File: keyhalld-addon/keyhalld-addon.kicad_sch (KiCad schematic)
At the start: 66 parts, among them J1 Conn_01x06_Pin, J2 USB_C_Receptacle_USB2.0_16P, J3 Conn_01x04_Pin, SW1 SW_Push, SW10 RST, SW2 SW_Push, SW3 SW_Push, SW4 SW_Push, SW5 SW_Push, SW6 SW_Push, SW7 SW_Push, SW8 SW_Push, SW9 BOOT, U1 TLV1117-33, U2 RP2350A, U3 USBLC6-2SC6, U4 ER_OLEDM0.91_1x-I2C, Y1 12MHz

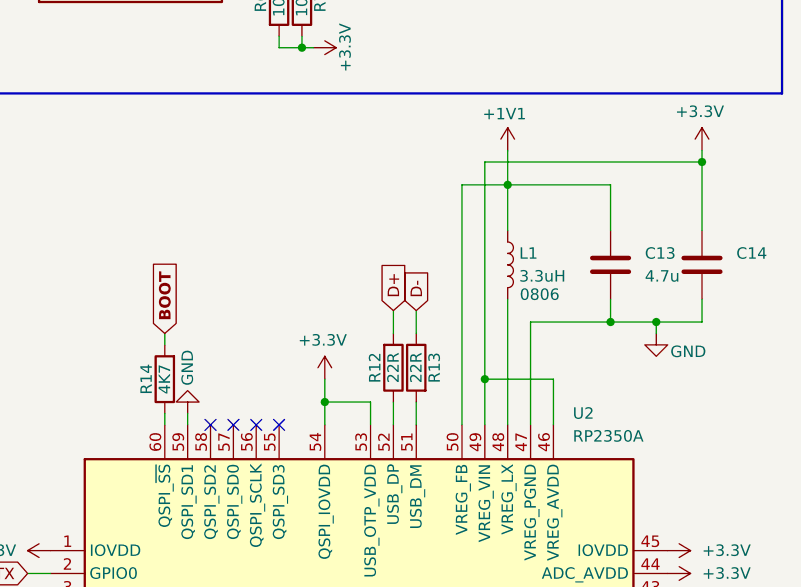
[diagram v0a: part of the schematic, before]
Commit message: routed pcb for addon board
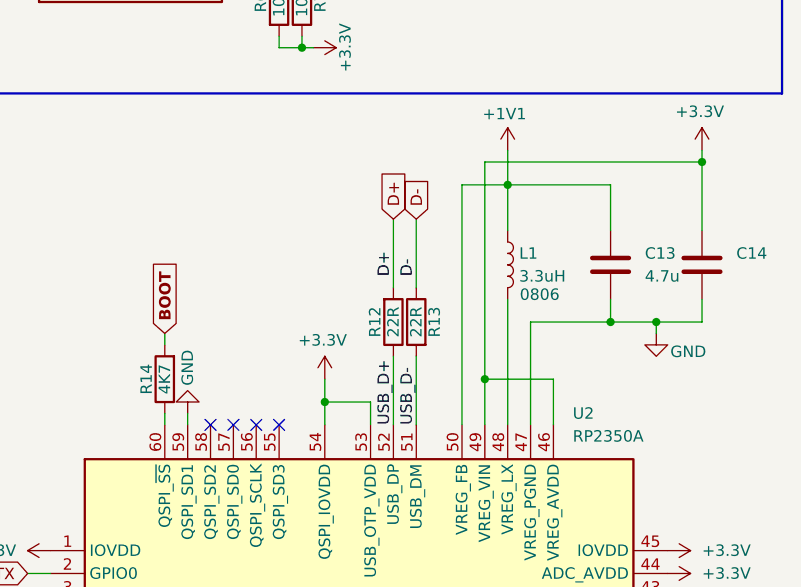
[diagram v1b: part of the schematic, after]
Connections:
- net USB_D-: now reaches R13.2, U2.51 (USB_DM)
- net USB_D+: now reaches R12.1, U2.52 (USB_DP)
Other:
- moved on the sheet: R12, R13
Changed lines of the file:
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@@
 	(wire
 		(pts
-			(xy 222.25 74.93) (xy 222.25 77.47)
+			(xy 222.25 64.77) (xy 222.25 72.39)
 		)
 		(stroke
@@
 	(wire
 		(pts
-			(xy 222.25 85.09) (xy 222.25 87.63)
+			(xy 222.25 80.01) (xy 222.25 87.63)
 		)
 		(stroke
@@
 	(wire
 		(pts
-			(xy 224.79 85.09) (xy 224.79 87.63)
+			(xy 224.79 80.01) (xy 224.79 87.63)
 		)
 		(stroke
@@
 	(wire
 		(pts
-			(xy 224.79 74.93) (xy 224.79 77.47)
+			(xy 224.79 64.77) (xy 224.79 72.39)
 		)
 		(stroke
@@
 		)
 	)
+	(label "USB_D-"
+		(at 224.79 87.63 90)
+		(effects
+			(font
+				(size 1.27 1.27)
+			)
+			(justify left bottom)
+		)
+	)
 	(label "CONN_D-"
 		(at 88.9 140.97 0)
@@
 		)
 	)
+	(label "USB_D+"
+		(at 222.25 87.63 90)
+		(effects
+			(font
+				(size 1.27 1.27)
+			)
+			(justify left bottom)
+		)
+	)
 	(label "CONN_D+"
 		(at 88.9 143.51 0)
@@
 		)
 	)
+	(label "D+"
+		(at 222.25 71.12 90)
+		(effects
+			(font
+				(size 1.27 1.27)
+			)
+			(justify left bottom)
+		)
+	)
+	(label "D-"
+		(at 224.79 71.12 90)
+		(effects
+			(font
+				(size 1.27 1.27)
+			)
+			(justify left bottom)
+		)
+	)
 	(global_label "WS_LED"
 		(shape input)
@@
 	(global_label "D+"
 		(shape input)
-		(at 222.25 74.93 90)
+		(at 222.25 64.77 90)
 		(fields_autoplaced yes)
 		(effects
@@
 		)
 		(property "Intersheetrefs" "${INTERSHEET_REFS}"
-			(at 222.25 69.1024 90)
+			(at 222.25 58.9424 90)
 			(hide yes)
 			(show_name no)
@@
 	(global_label "D-"
 		(shape input)
-		(at 224.79 74.93 90)
+		(at 224.79 64.77 90)
 		(fields_autoplaced yes)
 		(effects
@@
 		)
 		(property "Intersheetrefs" "${INTERSHEET_REFS}"
-			(at 224.79 69.1024 90)
+			(at 224.79 58.9424 90)
 			(hide yes)
 			(show_name no)
@@
 	(symbol
 		(lib_id "Device:R")
-		(at 224.79 81.28 0)
+		(at 224.79 76.2 0)
 		(mirror y)
 		(unit 1)
@@
 		(dnp no)
 		(property "Reference" "R13"
-			(at 226.822 81.28 90)
+			(at 226.822 76.2 90)
 			(show_name no)
 			(do_not_autoplace no)
@@
 		)
 		(property "Value" "22R"
-			(at 224.79 81.28 90)
+			(at 224.79 76.2 90)
 			(show_name no)
 			(do_not_autoplace no)
@@
 		)
 		(property "Footprint" "Resistor_SMD:R_0603_1608Metric_Pad0.98x0.95mm_HandSolder"
-			(at 226.568 81.28 90)
+			(at 226.568 76.2 90)
 			(hide yes)
 			(show_name no)
@@
 		)
 		(property "Datasheet" ""
-			(at 224.79 81.28 0)
+			(at 224.79 76.2 0)
 			(hide yes)
 			(show_name no)
@@
 		)
 		(property "Description" "Resistor"
-			(at 224.79 81.28 0)
+			(at 224.79 76.2 0)
 			(hide yes)
 			(show_name no)
@@
 	(symbol
 		(lib_id "Device:R")
-		(at 222.25 81.28 0)
+		(at 222.25 76.2 0)
 		(mirror x)
 		(unit 1)
@@
 		(dnp no)
 		(property "Reference" "R12"
-			(at 220.218 81.28 90)
+			(at 220.218 76.2 90)
 			(show_name no)
 			(do_not_autoplace no)
@@
 		)
 		(property "Value" "22R"
-			(at 222.25 81.28 90)
+			(at 222.25 76.2 90)
 			(show_name no)
 			(do_not_autoplace no)
@@
 		)
 		(property "Footprint" "Resistor_SMD:R_0603_1608Metric_Pad0.98x0.95mm_HandSolder"
-			(at 220.472 81.28 90)
+			(at 220.472 76.2 90)
 			(hide yes)
 			(show_name no)
@@
 		)
 		(property "Datasheet" ""
-			(at 222.25 81.28 0)
+			(at 222.25 76.2 0)
 			(hide yes)
 			(show_name no)
@@
 		)
 		(property "Description" "Resistor"
-			(at 222.25 81.28 0)
+			(at 222.25 76.2 0)
 			(hide yes)
 			(show_name no)

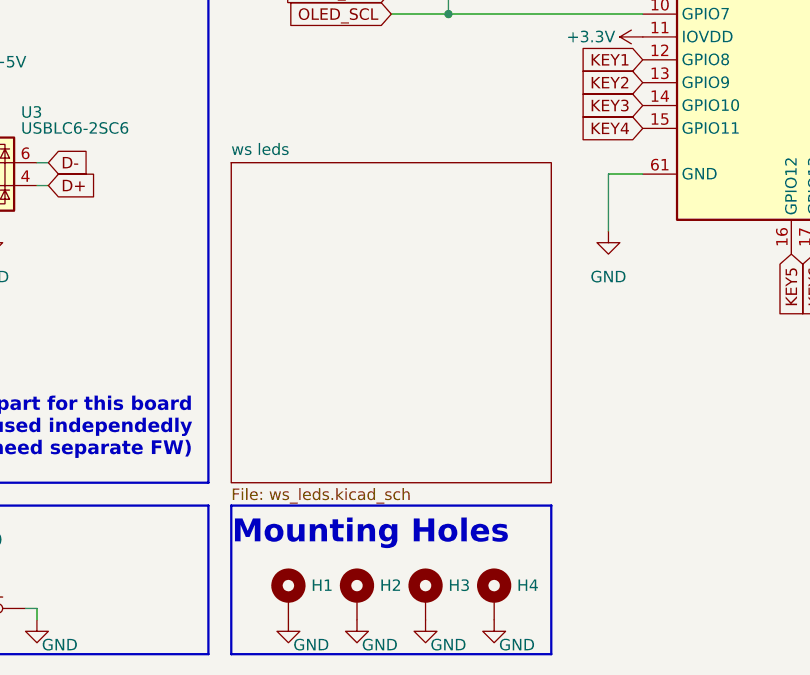
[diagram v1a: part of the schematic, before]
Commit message: stitching vias; one more hole
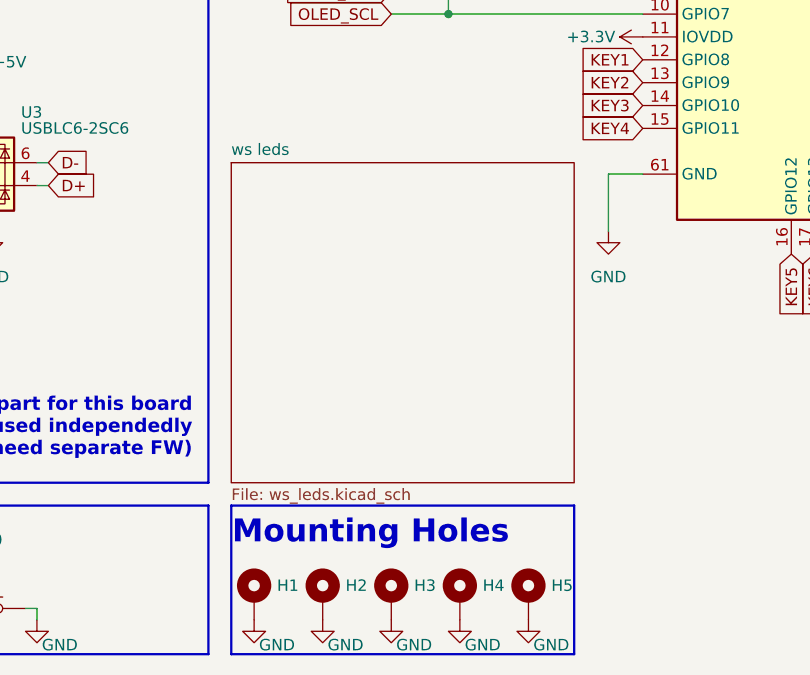
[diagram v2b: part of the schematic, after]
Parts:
- added H5: MountingHole_Pad, MountingHole:MountingHole_2.2mm_M2_DIN965_Pad, symbol Mechanical:MountingHole_Pad
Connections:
- net GND: now also H5.1
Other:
- moved on the sheet: H1, H2, H3, H4
